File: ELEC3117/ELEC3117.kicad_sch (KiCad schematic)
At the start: 8 parts, among them J1 USB_C_Receptacle_PowerOnly_6P, U1 AZ1117-3.3, U2 ESP32-WROOM-32D, U3 MCP73831-2-OT

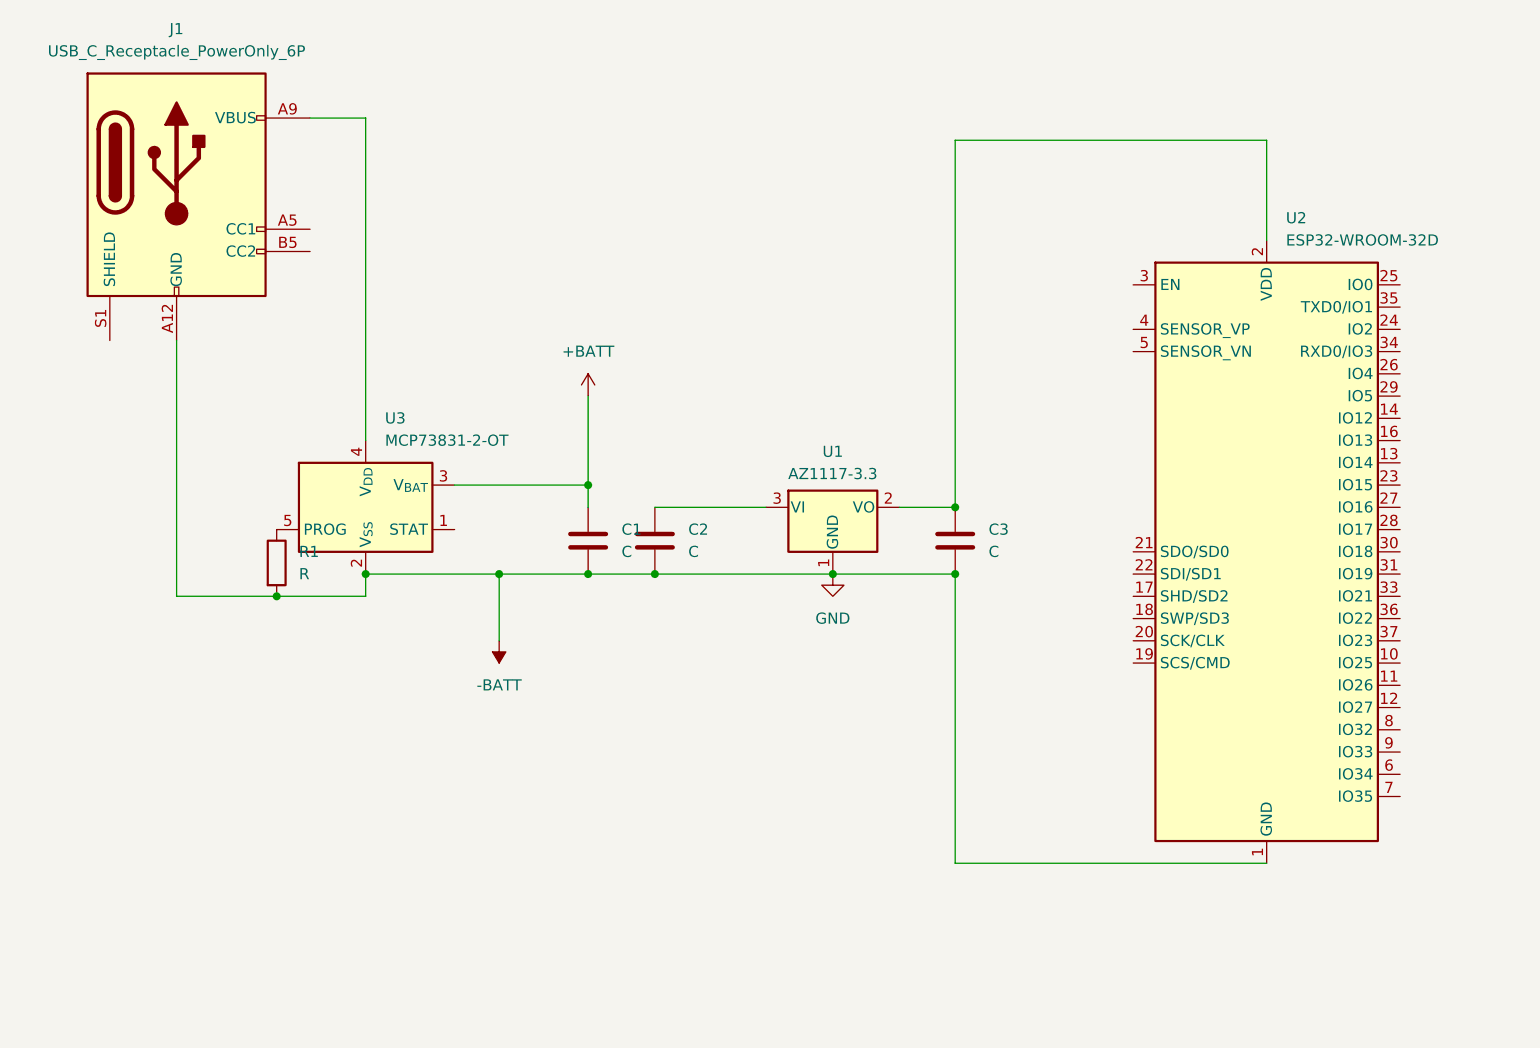
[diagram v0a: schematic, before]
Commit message: Add files via upload
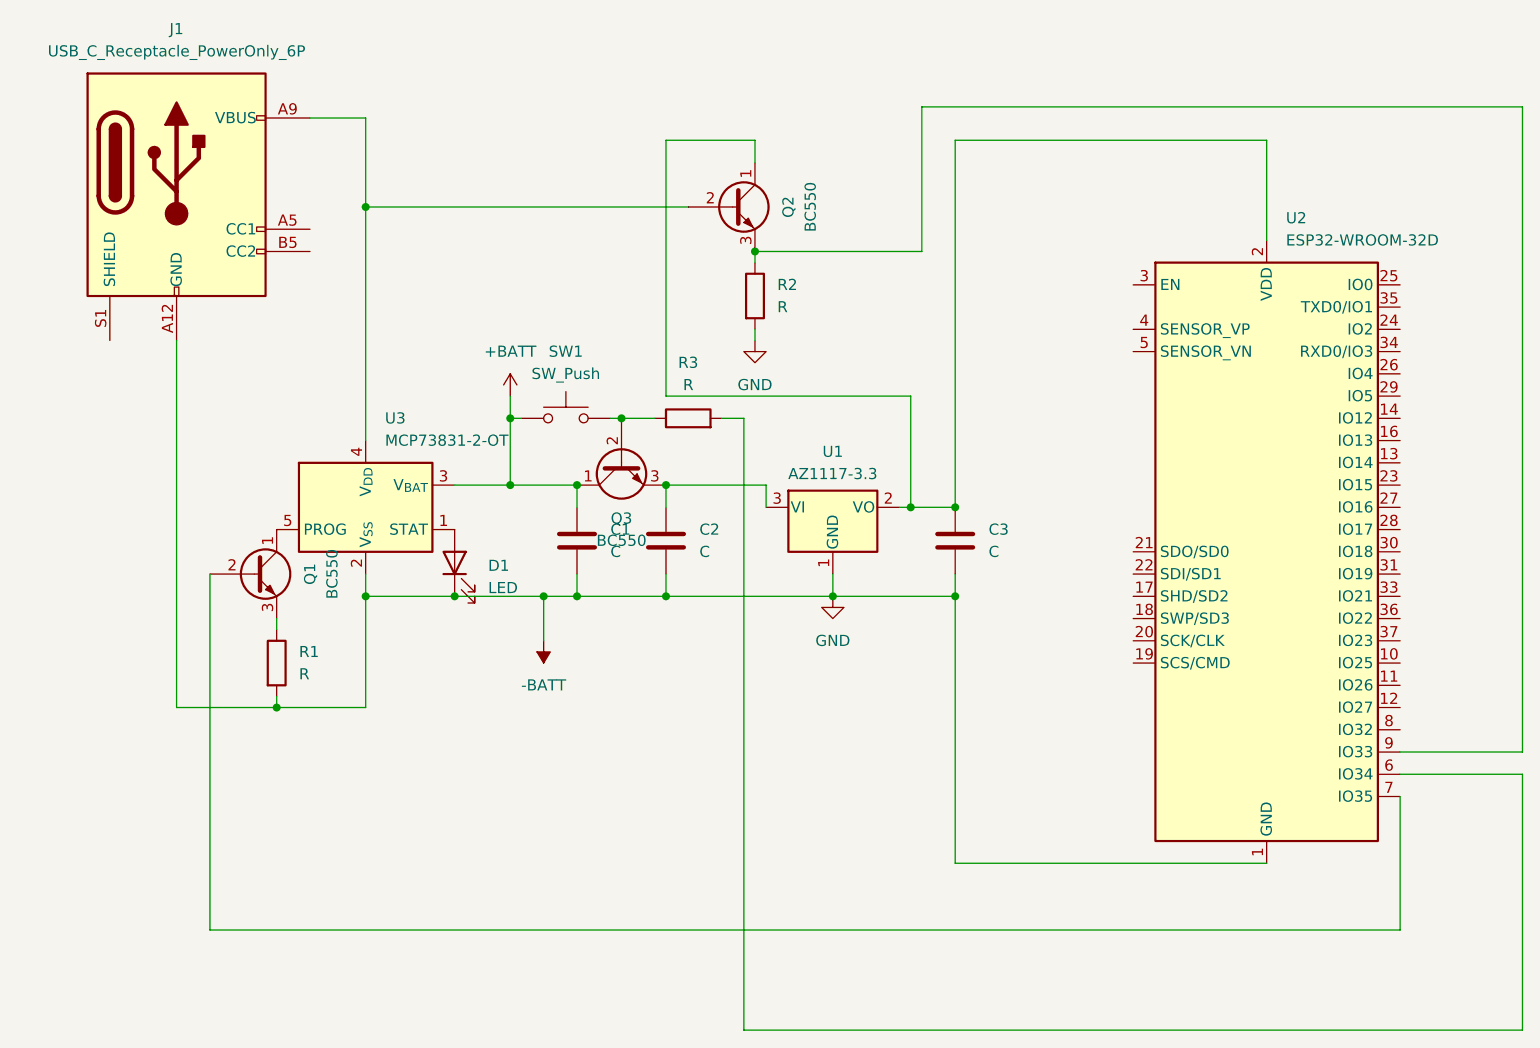
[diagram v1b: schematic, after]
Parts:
- added D1: LED, symbol Device:LED
- added Q1, Q2, Q3: BC550, Package_TO_SOT_THT:TO-92_Inline, symbol Transistor_BJT:BC550
- added R2, R3: R, symbol Device:R
- added SW1: SW_Push, symbol Switch:SW_Push
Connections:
- net +BATT: now also Q3.1 (C), SW1.1
- net -BATT: now also D1.1 (K), R2.2
- net at C3.1, U1.2 (VO), U2.2 (VDD): now also Q2.1 (C)
- net at U2.6 (IO34): now also R3.2
- net at U2.7 (IO35): now also Q1.2 (B)
- net at U2.9 (IO33): now also Q2.3 (E), R2.1
- net at J1.A9 (VBUS), J1.B9 (VBUS), U3.4 (V_{DD}): now also Q2.2 (B)
- net at C2.1, U1.3 (VI): now also Q3.3 (E)
- net at R1.1: now also Q1.3 (E); no longer U3.5 (PROG)
- net at U3.1 (STAT): now also D1.2 (A)
- new net: Q3.2 (B), R3.1, SW1.2
- new net: Q1.1 (C), U3.5 (PROG)
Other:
- moved on the sheet: C1, C2, R1
